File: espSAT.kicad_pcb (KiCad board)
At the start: 2 copper layers, 43 parts, among them J1 Micro_SD_Card_Det2, J2 Prog, J3 C5, J4 C1, J5 C2, J6 C6, Q1 IRFZ44N, Q2 IRFZ44N, Q3 IRFZ44N, U1 ESP32-WROOM-32, U2 INA219AxD, U3 AZ1117-3.3, U4 AZ1117-3.3, U5 INA219AxD, U6 INA219AxD

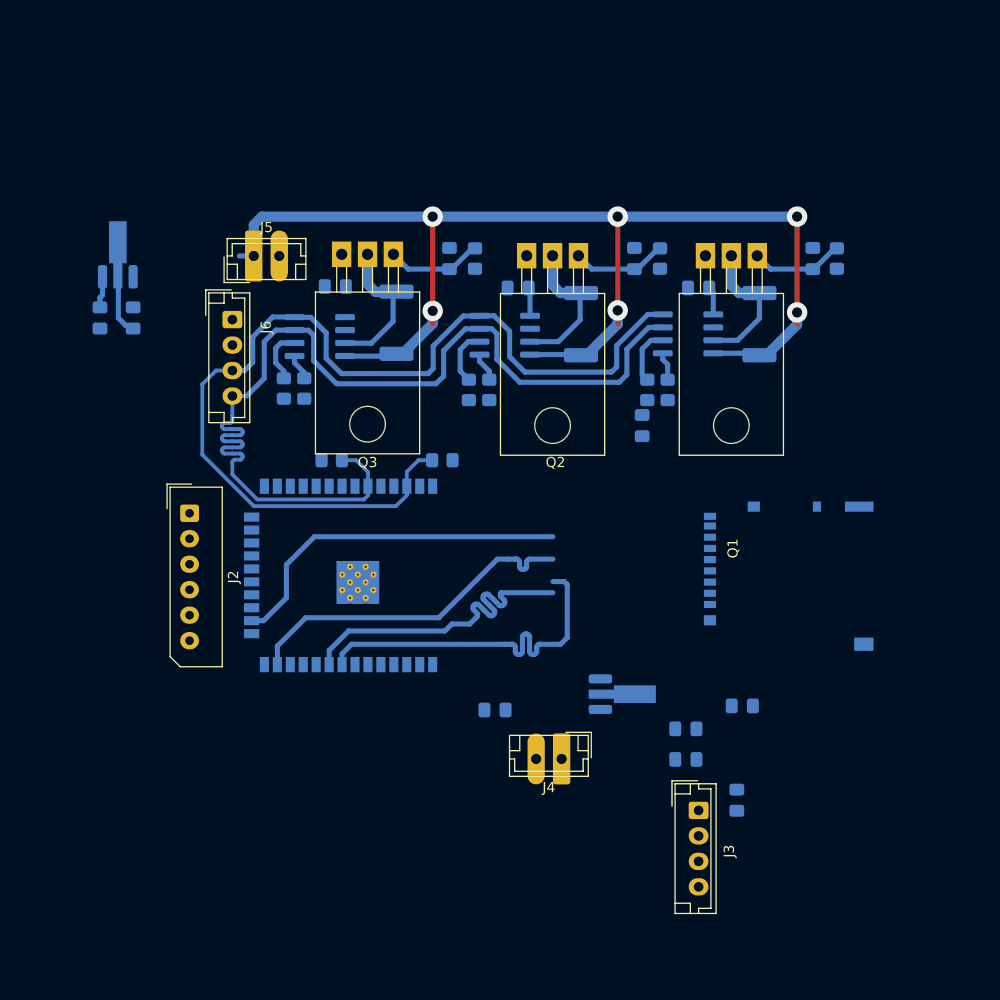
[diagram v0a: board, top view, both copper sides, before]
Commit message: v1
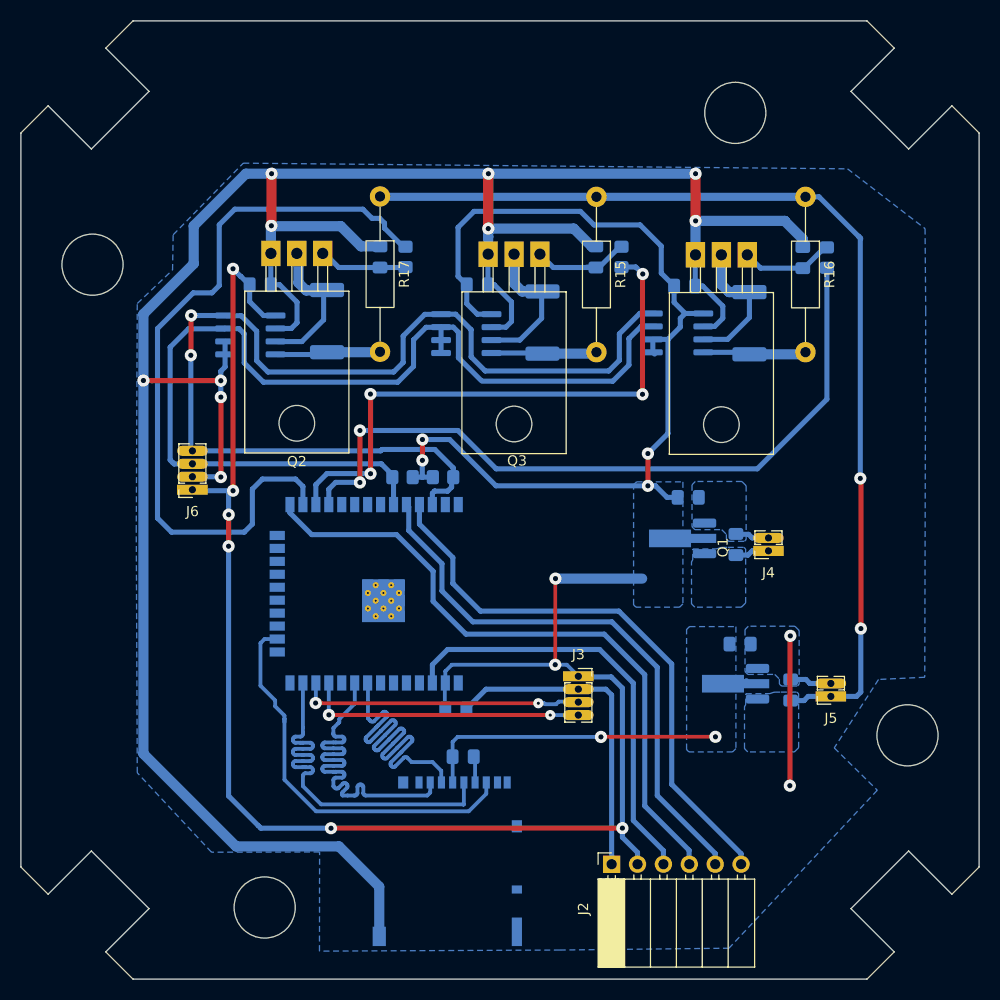
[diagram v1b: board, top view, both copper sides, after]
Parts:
- removed C2: 10μF, Capacitor_SMD:C_0805_2012Metric_Pad1.18x1.45mm_HandSolder
- removed C3: 22μF, Capacitor_SMD:C_0805_2012Metric_Pad1.18x1.45mm_HandSolder
- removed the Q3 at (134.6, 59.7)
- removed R10, R2, R3, R5, R6, R9: 10K, Resistor_SMD:R_0805_2012Metric_Pad1.20x1.40mm_HandSolder
- added Q2: IRLZ24, Package_TO_SOT_THT:TO-220-3_Horizontal_TabDown, F.Cu at (127.7, 59.6)
- added R15: R_US, Resistor_THT:R_Axial_DIN0207_L6.3mm_D2.5mm_P15.24mm_Horizontal, F.Cu at (154.5, 54.1)
- added R16: R_US, Resistor_THT:R_Axial_DIN0207_L6.3mm_D2.5mm_P15.24mm_Horizontal, F.Cu at (175.0, 54.1)
- added R17: R_US, Resistor_THT:R_Axial_DIN0207_L6.3mm_D2.5mm_P15.24mm_Horizontal, F.Cu at (133.3, 54.0)
- J2: footprint Connector_Molex:Molex_SPOX_5267-06A_1x06_P2.50mm_Vertical -> Connector_PinSocket_2.54mm:PinSocket_1x06_P2.54mm_Horizontal
- J3, J6: footprint Connector_JST:JST_EH_B4B-EH-A_1x04_P2.50mm_Vertical -> Connector_PinSocket_1.27mm:PinSocket_1x04_P1.27mm_Vertical
- J4, J5: footprint Connector_JST:JST_EH_B2B-EH-A_1x02_P2.50mm_Vertical -> Connector_PinSocket_1.27mm:PinSocket_1x02_P1.27mm_Vertical
- Q1: value IRFZ44N -> IRLZ24
- Q3: renamed from Q2; value IRFZ44N -> IRLZ24
- moved C5 77.0 mm to (173.6, 102.4), turned to 90 degrees
- moved U4 73.7 mm to (167.9, 101.8), turned to 180 degrees
- moved J5 71.2 mm to (177.5, 103.1), turned to 180 degrees
- moved C7 67.6 mm to (168.6, 97.9), turned to 0 degrees
- moved J2 53.8 mm to (156.0, 119.5), turned to 90 degrees
- moved J1 43.6 mm to (139.9, 119.2), turned to 180 degrees
- moved C15 36.9 mm to (141.4, 109.0), turned to 0 degrees
- moved J4 28.8 mm to (171.4, 88.8)
- moved C4 25.7 mm to (163.5, 83.5)
- moved C1 18.7 mm to (168.2, 88.2), turned to 90 degrees
- moved J3 17.7 mm to (152.7, 101.1), turned to 0 degrees
- moved J6 17.1 mm to (114.9, 82.8), turned to 180 degrees
- moved U3 16.2 mm to (162.7, 87.6), turned to 180 degrees
- moved C14 7.37 mm to (121.5, 62.7), turned to 0 degrees
- moved R13 7.14 mm to (135.5, 81.6), turned to 0 degrees
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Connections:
- J2 pad 2: IO0 -> 3.3V_{1}
- J2 pad 4: TXD0 -> IO0
- J2 pad 6: 3.3V_{1} -> TXD0
- J6 pad 3: SCL -> SDA
- J6 pad 4: SDA -> SCL
- R1 pad 1: V_{in2} -> Net-(U2-IN+)
- R11 pad 1: G3 -> G1
- R12 pad 1: V_{in2} -> Net-(U6-IN+)
- R4 pad 1: G1 -> G3
- R8 pad 1: V_{in2} -> Net-(U5-IN+)
- U1 pad 11: STEP -> DIR
- U1 pad 12: DIR -> STEP
- U2 pad 1: Net-(U2-A1) -> 3.3V_{1}
- U2 pad 2: Net-(U2-A0) -> 3.3V_{1}
- U2 pad 8: V_{in2} -> Net-(U2-IN+)
- U5 pad 1: 3.3V_{1} -> SDA
- U5 pad 2: Net-(U5-A0) -> SDA
- U5 pad 8: V_{in2} -> Net-(U5-IN+)
- U6 pad 1: Net-(U6-A1) -> GND
- U6 pad 2: 3.3V_{1} -> GND
- U6 pad 8: V_{in2} -> Net-(U6-IN+)
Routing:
- net GND: track 0.00 -> 308.6 mm, vias 0 -> 12
- net 3.3V_{1}: track 13.8 -> 256.4 mm, vias 0 -> 12
- net G1: track 0.00 -> 74.2 mm
- net G3: track 0.00 -> 73.0 mm, vias 0 -> 2
- net IO0: track 0.00 -> 64.3 mm
- net G2: track 0.00 -> 56.4 mm, vias 0 -> 4
- net TXD0: track 0.00 -> 56.3 mm
- net RXD0: track 0.00 -> 55.8 mm
- net EN: track 0.00 -> 42.5 mm
- net STEP: track 0.00 -> 28.1 mm, vias 0 -> 2
- net DIR: track 0.00 -> 27.6 mm, vias 0 -> 2
- net 3.3V_{2}: track 6.03 -> 30.0 mm, vias 0 -> 2
- net V_{in2}: track 124.4 -> 100.9 mm, vias 6 -> 2
- net Net-(U2-IN+): track 0.00 -> 10.8 mm
- net Net-(U5-IN+): track 0.00 -> 10.3 mm
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- added copper zone on B.Cu, net 3.3V_{1}
- added copper zone on B.Cu, net 3.3V_{2}
- added copper zone on B.Cu, net GND
- added copper zone on B.Cu, net V_{in1}
- added copper zone on B.Cu, net V_{in2}
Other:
- board outline added: 94 x 94 mm
